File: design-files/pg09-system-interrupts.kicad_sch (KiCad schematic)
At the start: 12 parts, among them Q401 2N7000, U401 W65C21, U402 GAL22V10, U403 GAL22V10, U404 GAL22V10

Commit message: Specify a physically smaller bypass cap.
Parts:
- C201, C202, C203: footprint Capacitor_THT:C_Disc_D6.0mm_W4.4mm_P5.00mm -> Capacitor_THT:C_Disc_D3.8mm_W2.6mm_P2.50mm
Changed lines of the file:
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@@
       (effects (font (size 1.27 1.27)) (justify left))
     )
-    (property "Footprint" "Capacitor_THT:C_Disc_D6.0mm_W4.4mm_P5.00mm" (at 223.52 137.16 0)
+    (property "Footprint" "Capacitor_THT:C_Disc_D3.8mm_W2.6mm_P2.50mm" (at 223.52 137.16 0)
       (effects (font (size 1.27 1.27)) hide)
     )
@@
       (effects (font (size 1.27 1.27)) (justify left))
     )
-    (property "Footprint" "Capacitor_THT:C_Disc_D6.0mm_W4.4mm_P5.00mm" (at 243.84 137.16 0)
+    (property "Footprint" "Capacitor_THT:C_Disc_D3.8mm_W2.6mm_P2.50mm" (at 243.84 137.16 0)
       (effects (font (size 1.27 1.27)) hide)
     )
@@
       (effects (font (size 1.27 1.27)) (justify left))
     )
-    (property "Footprint" "Capacitor_THT:C_Disc_D6.0mm_W4.4mm_P5.00mm" (at 233.68 137.16 0)
+    (property "Footprint" "Capacitor_THT:C_Disc_D3.8mm_W2.6mm_P2.50mm" (at 233.68 137.16 0)
       (effects (font (size 1.27 1.27)) hide)
     )
@@
       (effects (font (size 1.27 1.27)) (justify left))
     )
-    (property "Footprint" "Capacitor_THT:C_Disc_D6.0mm_W4.4mm_P5.00mm" (at 254 137.16 0)
-      (effects (font (size 1.27 1.27)) hide)
-    )
+    (property "Footprint" "Capacitor_THT:C_Disc_D3.8mm_W2.6mm_P2.50mm" (at 254 137.16 0)
+      (effects (font (size 1.27 1.27)) hide)
+    )

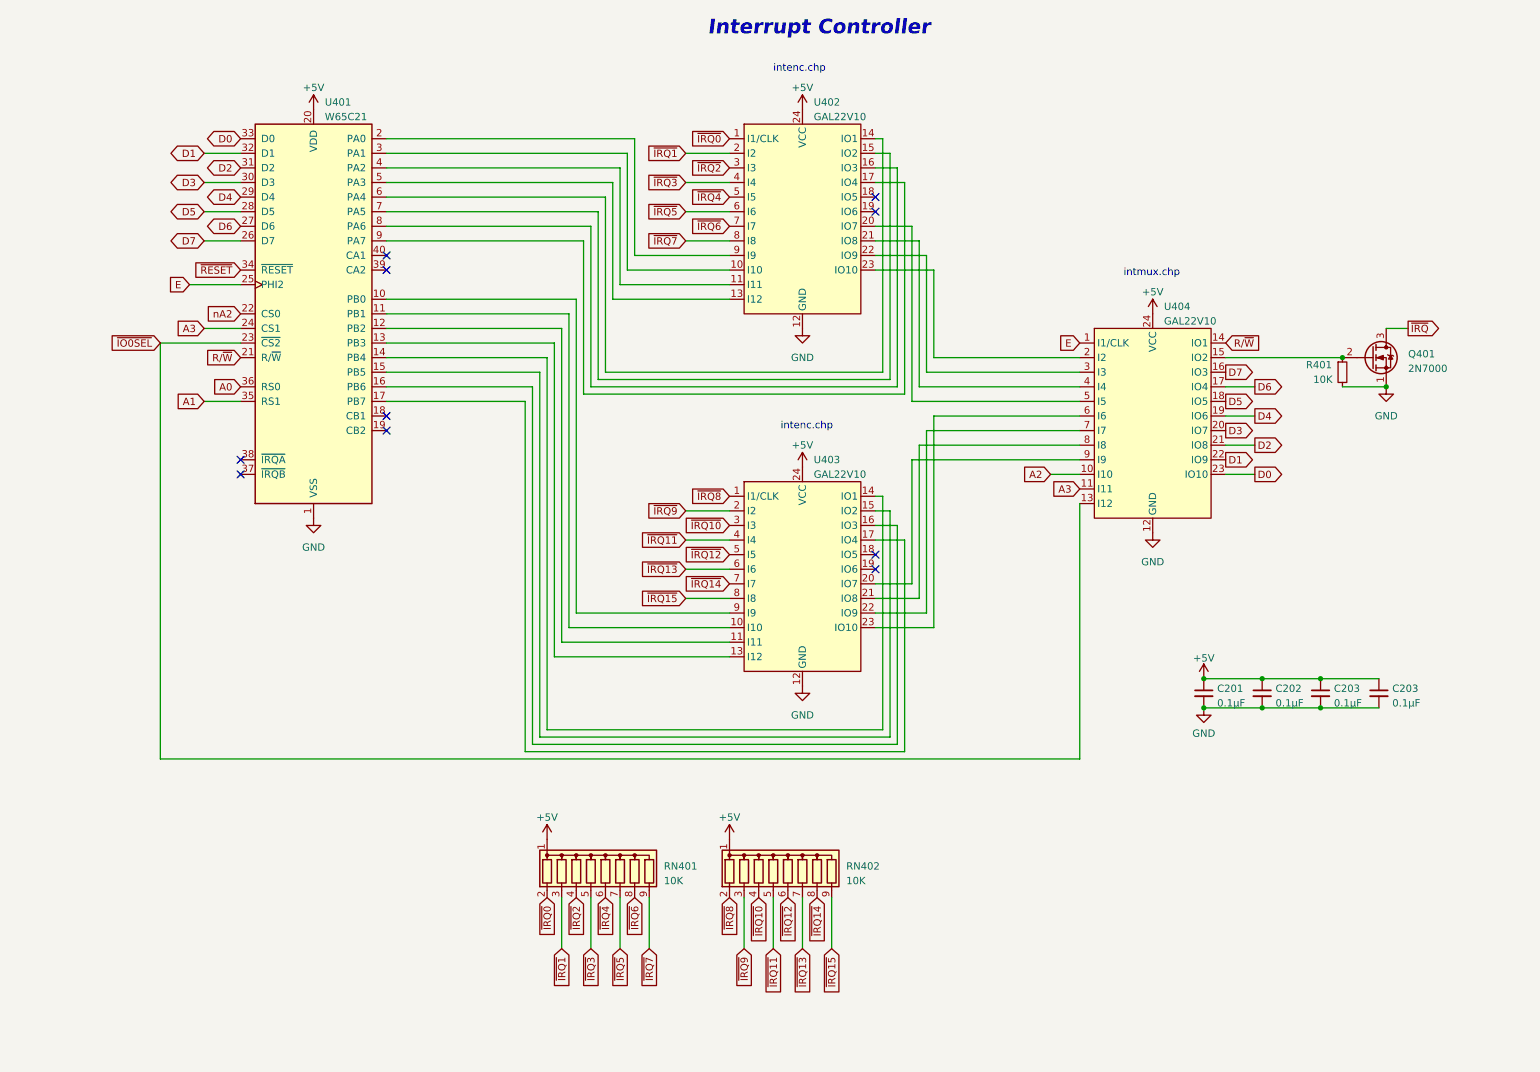
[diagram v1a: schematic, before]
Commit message: Integrate the auto-vectoring interrupt controller.
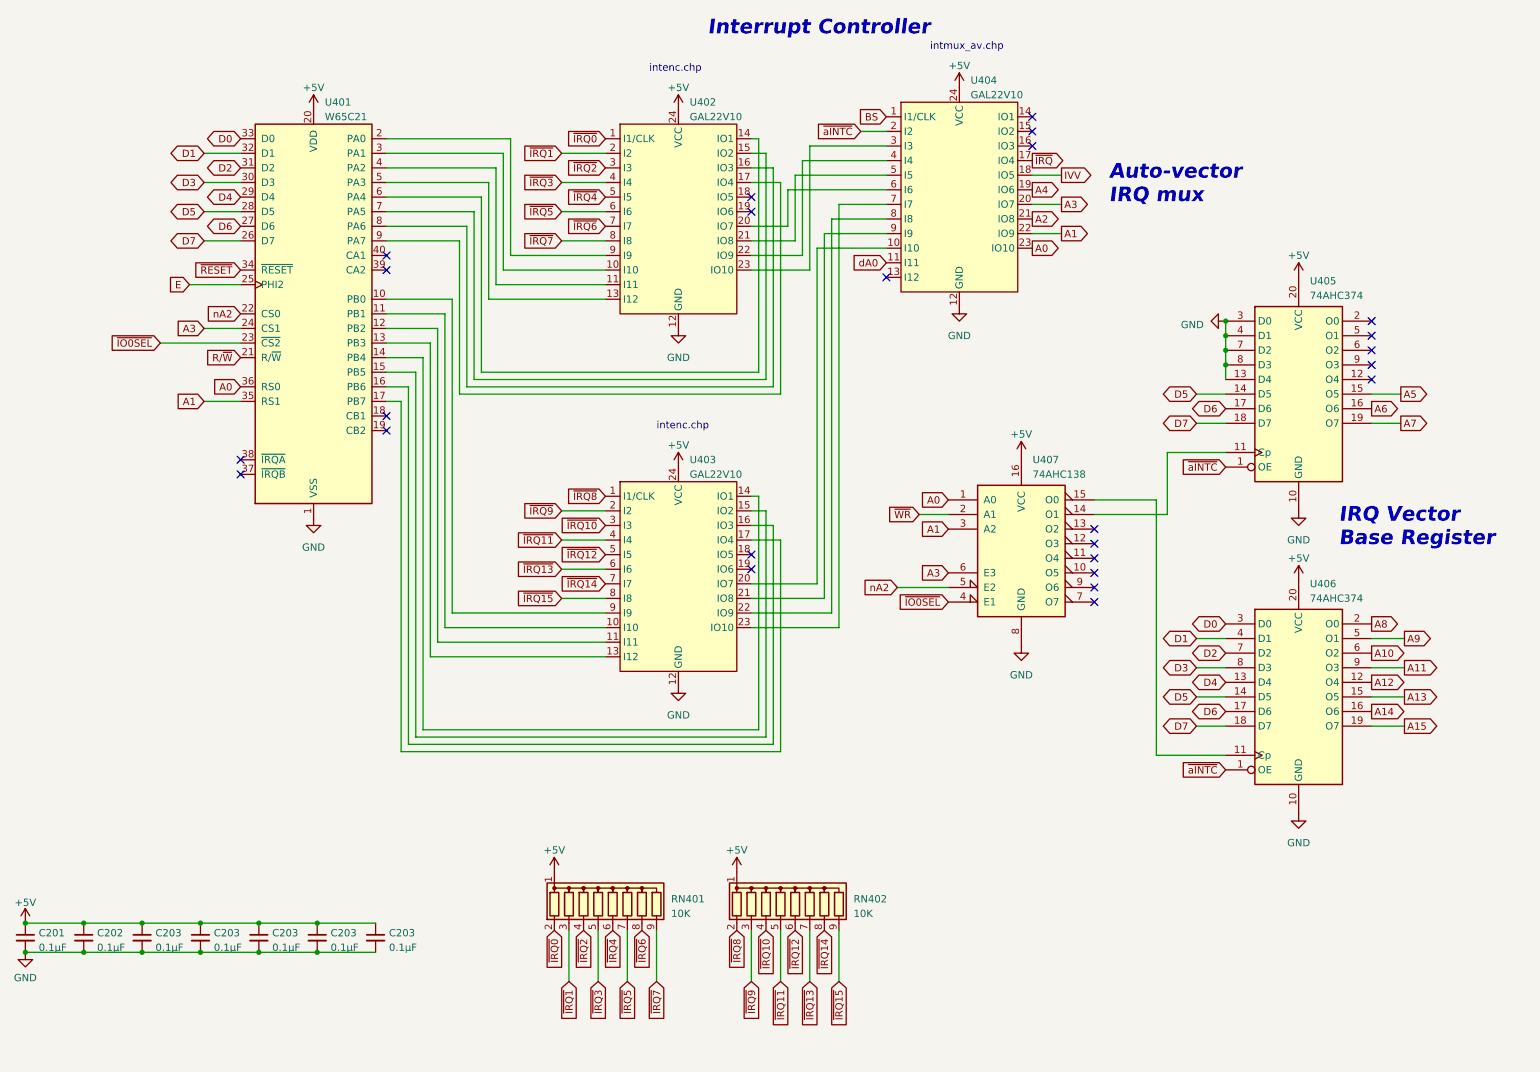
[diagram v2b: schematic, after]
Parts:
- removed Q401: 2N7000, Package_TO_SOT_THT:TO-92_Inline, symbol Transistor_FET:2N7000
- removed R401: 10K, Resistor_THT:R_Axial_DIN0207_L6.3mm_D2.5mm_P7.62mm_Horizontal, symbol Device:R_Small
- added C203 (x3): 0.1µF, Capacitor_THT:C_Disc_D3.8mm_W2.6mm_P2.50mm, symbol Device:C_Small
- added U405, U406: 74AHC374, symbol 74xx:74AHC374
- added U407: 74AHC138, symbol 74xx:74LS138
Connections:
- net +5V: now also C203.1, C203.1, C203.1, U405.20 (VCC), U406.20 (VCC), U407.16 (VCC)
- net A0: now also U404.23 (IO10), U407.1 (A0)
- net A1: now also U404.22 (IO9), U407.3 (A2)
- net A2: now also U404.21 (IO8); no longer U404.10 (I10)
- net A3: now also U404.20 (IO7), U407.6 (E3); no longer U404.11 (I11)
- net D0: now also U406.3 (D0); no longer U404.23 (IO10)
- net D1: now also U406.4 (D1); no longer U404.22 (IO9)
- net D2: now also U406.7 (D2); no longer U404.21 (IO8)
- net D3: now also U406.8 (D3); no longer U404.20 (IO7)
- net D4: now also U406.13 (D4); no longer U404.19 (IO6)
- net D5: now also U405.14 (D5), U406.14 (D5); no longer U404.18 (IO5)
- net D6: now also U405.17 (D6), U406.17 (D6); no longer U404.17 (IO4)
- net D7: now also U405.18 (D7), U406.18 (D7); no longer U404.16 (IO3)
- net E: no longer U404.1 (I1/CLK)
- net GND: now also C203.2, C203.2, C203.2, U405.10 (GND), U405.13 (D4), U405.3 (D0), U405.4 (D1), U405.7 (D2), U405.8 (D3), U406.10 (GND), U407.8 (GND)
- net R/~{W}: no longer U404.14 (IO1)
- net nA2: now also U407.5 (E2)
- net ~{IO0SEL}: now also U407.4 (E1); no longer U404.13 (I12)
- net ~{IRQ}: now also U404.17 (IO4)
- net at U402.23 (IO10): now also U404.3 (I3); no longer U404.2 (I2)
- net at U402.22 (IO9): now also U404.4 (I4); no longer U404.3 (I3)
- net at U402.21 (IO8): now also U404.5 (I5); no longer U404.4 (I4)
- net at U402.20 (IO7): now also U404.6 (I6); no longer U404.5 (I5)
- net at U403.23 (IO10): now also U404.7 (I7); no longer U404.6 (I6)
- net at U403.22 (IO9): now also U404.8 (I8); no longer U404.7 (I7)
- net at U403.21 (IO8): now also U404.9 (I9); no longer U404.8 (I8)
- net at U403.20 (IO7): now also U404.10 (I10); no longer U404.9 (I9)
- new net: U406.11 (Cp), U407.15 (O0)
- new net: U405.11 (Cp), U407.14 (O1)
- new net A10: U406.6 (O2)
- new net A11: U406.9 (O3)
- new net A12: U406.12 (O4)
- new net A13: U406.15 (O5)
- new net A14: U406.16 (O6)
- new net A15: U406.19 (O7)
- new net A4: U404.19 (IO6)
- new net A5: U405.15 (O5)
- new net A6: U405.16 (O6)
- new net A7: U405.19 (O7)
- new net A8: U406.2 (O0)
- new net A9: U406.5 (O1)
- new net BS: U404.1 (I1/CLK)
- new net IVV: U404.18 (IO5)
- new net dA0: U404.11 (I11)
- new net ~{WR}: U407.2 (A1)
- new net ~{aINTC}: U404.2 (I2), U405.1 (OE), U406.1 (OE)
- no-connect marks 10 -> 25
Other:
- note added: "Auto-vector IRQ mux"
- note added: "IRQ Vector Base Register"
- note added: "intmux_av.chp"
- note removed: "intmux.chp"
- moved on the sheet: C201, C202, C203, RN401, RN402, U402, U403, U404

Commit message: WIP re-laying out PCB.
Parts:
- U405, U406: footprint (none) -> Package_DIP:DIP-20_W7.62mm_Socket
- U407: footprint (none) -> Package_DIP:DIP-16_W7.62mm_Socket
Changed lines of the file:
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@@
       (effects (font (size 1.27 1.27)) (justify left))
     )
-    (property "Footprint" "" (at 240.03 137.795 0)
+    (property "Footprint" "Package_DIP:DIP-20_W7.62mm_Socket" (at 240.03 137.795 0)
       (effects (font (size 1.27 1.27)) hide)
     )
@@
       (effects (font (size 1.27 1.27)) (justify left))
     )
-    (property "Footprint" "" (at 240.03 85.09 0)
+    (property "Footprint" "Package_DIP:DIP-20_W7.62mm_Socket" (at 240.03 85.09 0)
       (effects (font (size 1.27 1.27)) hide)
     )
@@
       (effects (font (size 1.27 1.27)) (justify left))
     )
-    (property "Footprint" "" (at 191.77 111.125 0)
-      (effects (font (size 1.27 1.27)) hide)
-    )
+    (property "Footprint" "Package_DIP:DIP-16_W7.62mm_Socket" (at 191.77 111.125 0)
+      (effects (font (size 1.27 1.27)) hide)
+    )
